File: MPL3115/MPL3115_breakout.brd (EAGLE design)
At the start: 15.2 x 11.2 mm, 2 parts

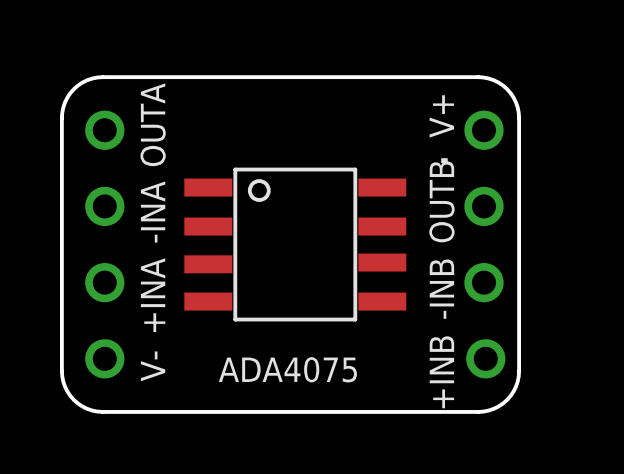
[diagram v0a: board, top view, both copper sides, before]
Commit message: Update new meme.
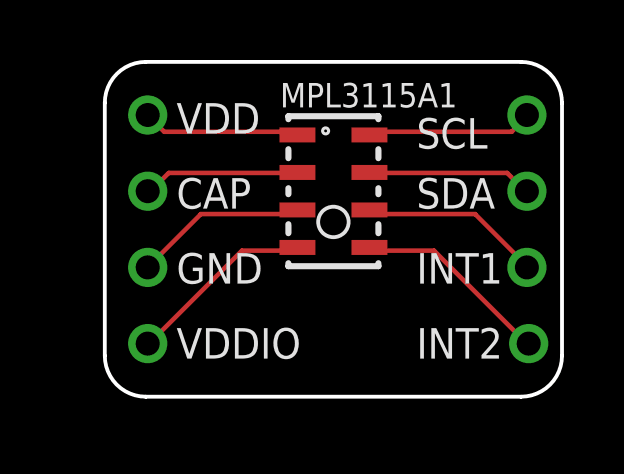
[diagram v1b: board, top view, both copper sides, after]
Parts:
- removed .: ADA4075, FaBo-Opamp:SOIC(NARROW)-8
- removed U$3: 8PIN, FaBo-Breakout:8PIN
- added MPL3115A1: FS-MPL3115A2, FaBo-Mems:FREESCALE-MPL3115A2
- added U$1: 8PIN, FaBo-Breakout:8PIN
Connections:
- removed net 1: ..1, U$3.1
- removed net 2: ..2, U$3.2
- removed net 3: ..3, U$3.3
- removed net 4: ..4, U$3.4
- removed net 5: ..5, U$3.5
- removed net 6: ..6, U$3.6
- removed net 7: ..7, U$3.7
- removed net 8: ..8, U$3.8
- new net CAP: MPL3115A1.2, U$1.2
- new net GND: MPL3115A1.3, U$1.3
- new net INT1: MPL3115A1.6, U$1.6
- new net INT2: MPL3115A1.5, U$1.5
- new net SCL: MPL3115A1.8, U$1.8
- new net SDA: MPL3115A1.7, U$1.7
- new net VDD: MPL3115A1.1, U$1.1
- new net VDDIO: MPL3115A1.4, U$1.4
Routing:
- net INT2: track 0.00 -> 6.67 mm
- net VDDIO: track 0.00 -> 6.35 mm
- net INT1: track 0.00 -> 6.13 mm
- net GND: track 0.00 -> 5.85 mm
- net SCL: track 0.00 -> 5.59 mm
- net SDA: track 0.00 -> 5.51 mm
- net VDD: track 0.00 -> 5.31 mm
- net CAP: track 0.00 -> 5.25 mm
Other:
- board text added: "CAP"
- board text added: "GND"
- board text added: "INT1"
- board text added: "INT2"
- board text added: "SCL"
- board text added: "SDA"
- board text added: "VDD"
- board text added: "VDDIO"
- board text removed: "+INA"
- board text removed: "+INB"
- board text removed: "-INA"
- board text removed: "-INB"
- board text removed: "ADA4075"
- board text removed: "OUTA"
- board text removed: "OUTB"
- board text removed: "V+"
- board text removed: "V-"
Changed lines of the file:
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@@
 <setting verticaltext="up"/>
 </settings>
-<grid distance="0.25" unitdist="mm" unit="mm" style="lines" multiple="1" display="yes" altdistance="0.025" altunitdist="inch" altunit="inch"/>
+<grid distance="0.5" unitdist="mm" unit="mm" style="lines" multiple="1" display="yes" altdistance="0.025" altunitdist="inch" altunit="inch"/>
 <layers>
 <layer number="1" name="Top" color="4" fill="1" visible="yes" active="yes"/>
@@
 <layer number="49" name="Reference" color="7" fill="1" visible="yes" active="yes"/>
 <layer number="50" name="dxf" color="7" fill="1" visible="no" active="no"/>
-<layer number="51" name="tDocu" color="14" fill="1" visible="yes" active="yes"/>
+<layer number="51" name="tDocu" color="7" fill="1" visible="yes" active="yes"/>
 <layer number="52" name="bDocu" color="7" fill="1" visible="yes" active="yes"/>
 <layer number="53" name="tGND_GNDA" color="7" fill="9" visible="no" active="no"/>
@@
 <layer number="154" name="FabDoc2" color="2" fill="1" visible="no" active="no"/>
 <layer number="155" name="FabDoc3" color="7" fill="15" visible="no" active="no"/>
-<layer number="160" name="O_Dim" color="12" fill="11" visible="yes" active="yes"/>
 <layer number="199" name="Contour" color="7" fill="1" visible="yes" active="yes"/>
-<layer number="200" name="200bmp" color="1" fill="10" visible="yes" active="yes"/>
+<layer number="200" name="200bmp" color="1" fill="10" visible="no" active="yes"/>
 <layer number="201" name="201bmp" color="2" fill="1" visible="no" active="no"/>
 <layer number="202" name="202bmp" color="3" fill="1" visible="no" active="no"/>
@@
 <board>
 <plain>
-<text x="3.794" y="1.262" size="0.8128" layer="21">ADA4075</text>
-<text x="2.016" y="8.398" size="0.8128" layer="21" rot="R90">OUTA</text>
-<text x="2.016" y="5.858" size="0.8128" layer="21" rot="R90">-INA</text>
-<text x="2.016" y="2.818" size="0.8128" layer="21" rot="R90">+INA</text>
-<text x="11.64" y="9.398" size="0.8128" layer="21" rot="R90">V+</text>
-<text x="11.644" y="5.858" size="0.8128" layer="21" rot="R90">OUTB</text>
-<text x="11.644" y="3.318" size="0.8128" layer="21" rot="R90">-INB</text>
-<text x="11.644" y="0.278" size="0.8128" layer="21" rot="R90">+INB</text>
-<text x="2.016" y="1.278" size="0.8128" layer="21" rot="R90">V-</text>
+<text x="2.39" y="9.54" size="1.016" layer="21">VDD</text>
+<text x="2.39" y="7.04" size="1.016" layer="21">CAP</text>
+<text x="2.39" y="4.54" size="1.016" layer="21">GND</text>
+<text x="2.39" y="2.04" size="1.016" layer="21">VDDIO</text>
+<text x="10.39" y="2.04" size="1.016" layer="21">INT2</text>
+<text x="10.39" y="4.54" size="1.016" layer="21">INT1</text>
+<text x="10.39" y="7.04" size="1.016" layer="21">SDA</text>
+<text x="10.39" y="9.04" size="1.016" layer="21">SCL</text>
 </plain>
 <attributes>
@@
 </class>
 </classes>
-<designrules name="Elecrow_2-layer_eagle_rule">
+<designrules name="SeeedStudio_2layer_DRU_no_angle_20140221">
 <description language="de">&lt;b&gt;EAGLE Design Rules&lt;/b&gt;
 &lt;p&gt;
@@
 necessary adjustments and save your customized
 design rules under a new name.</description>
-<description language="zh">&lt;b&gt;Elecrow EAGLE Design Rules&lt;/b&gt;
+<description language="zh">&lt;b&gt;Seeed Studio EAGLE Design Rules&lt;/b&gt;
 </description>
 <param name="layerSetup" value="(1*16)"/>
-<param name="mtCopper" value="0.035mm 0.035mm 0.035mm 0.035mm 0.035mm 0.035mm 0.035mm 0.035mm 0.035mm 0.035mm 0.035mm 0.035mm 0.035mm 0.035mm 0.035mm 0.035mm"/>
-<param name="mtIsolate" value="1.5mm 0.15mm 0.2mm 0.15mm 0.2mm 0.15mm 0.2mm 0.15mm 0.2mm 0.15mm 0.2mm 0.15mm 0.2mm 0.15mm 0.2mm"/>
+<param name="mtCopper" value="0.035mm 0.0175mm 0.035mm 0.035mm 0.035mm 0.035mm 0.035mm 0.035mm 0.035mm 0.035mm 0.035mm 0.035mm 0.035mm 0.035mm 0.0175mm 0.035mm"/>
+<param name="mtIsolate" value="1.5mm 1.1mm 0.2mm 0.15mm 0.2mm 0.15mm 0.2mm 0.15mm 0.2mm 0.15mm 0.2mm 0.15mm 0.2mm 0.15mm 0.2mm"/>
 <param name="mdWireWire" value="6mil"/>
 <param name="mdWirePad" value="6mil"/>
@@
 </autorouter>
 <elements>
-<element name="U$3" library="FaBo-Breakout" package="8PIN" value="8PIN" x="7.46" y="5.842"/>
-<element name="." library="FaBo-Opamp" package="SOIC(NARROW)-8" value="ADA4075" x="6.35" y="5.842" rot="R270"/>
+<element name="MPL3115A1" library="FaBo-Mems" package="FREESCALE-MPL3115A2" value="FS-MPL3115A2" x="7.62" y="7.62"/>
+<element name="U$1" library="FaBo-Breakout" package="8PIN" value="8PIN" x="8.89" y="6.35"/>
 </elements>
 <signals>
-<signal name="1">
-<contactref element="U$3" pad="1"/>
-<contactref element="." pad="1"/>
-<wire x1="3.45" y1="7.742" x2="0" y2="9.652" width="0" layer="19" extent="1-1"/>
-</signal>
-<signal name="2">
-<contactref element="U$3" pad="2"/>
-<contactref element="." pad="2"/>
-<wire x1="0" y1="7.112" x2="3.45" y2="6.442" width="0" layer="19" extent="1-1"/>
-</signal>
-<signal name="3">
-<contactref element="U$3" pad="3"/>
-<contactref element="." pad="3"/>
-<wire x1="0" y1="4.572" x2="3.45" y2="5.182" width="0" layer="19" extent="1-1"/>
-</signal>
-<signal name="4">
-<contactref element="U$3" pad="4"/>
-<contactref element="." pad="4"/>
-<wire x1="0" y1="2.032" x2="3.45" y2="3.942" width="0" layer="19" extent="1-1"/>
-</signal>
-<signal name="8">
-<contactref element="U$3" pad="8"/>
-<contactref element="." pad="8"/>
-<wire x1="9.25" y1="7.742" x2="12.64" y2="9.652" width="0" layer="19" extent="1-1"/>
-</signal>
-<signal name="7">
-<contactref element="U$3" pad="7"/>
-<contactref element="." pad="7"/>
-<wire x1="9.25" y1="6.442" x2="12.64" y2="7.112" width="0" layer="19" extent="1-1"/>
-</signal>
-<signal name="6">
-<contactref element="U$3" pad="6"/>
-<contactref element="." pad="6"/>
-<wire x1="9.25" y1="5.242" x2="12.64" y2="4.572" width="0" layer="19" extent="1-1"/>
-</signal>
-<signal name="5">
-<contactref element="U$3" pad="5"/>
-<contactref element="." pad="5"/>
-<wire x1="12.7" y1="2.032" x2="9.25" y2="3.942" width="0" layer="19" extent="1-1"/>
+<signal name="VDD">
+<contactref element="U$1" pad="1"/>
+<contactref element="MPL3115A1" pad="1"/>
+<wire x1="1.9812" y1="9.6012" x2="6.4008" y2="9.6012" width="0.1524" layer="1"/>
+<wire x1="1.524" y1="10.0584" x2="1.9812" y2="9.6012" width="0.1524" layer="1"/>
+<wire x1="6.4008" y1="9.6012" x2="6.42" y2="9.495" width="0.1524" layer="1"/>
+<wire x1="1.524" y1="10.0584" x2="1.43" y2="10.16" width="0.1524" layer="1"/>
+</signal>
+<signal name="CAP">
+<contactref element="U$1" pad="2"/>
+<contactref element="MPL3115A1" pad="2"/>
+<wire x1="2.1336" y1="8.2296" x2="6.4008" y2="8.2296" width="0.1524" layer="1"/>
+<wire x1="1.524" y1="7.62" x2="2.1336" y2="8.2296" width="0.1524" layer="1"/>
+<wire x1="6.4008" y1="8.2296" x2="6.42" y2="8.245" width="0.1524" layer="1"/>
+<wire x1="1.524" y1="7.62" x2="1.43" y2="7.62" width="0.1524" layer="1"/>
+</signal>
+<signal name="GND">
+<contactref element="U$1" pad="3"/>
+<contactref element="MPL3115A1" pad="3"/>
+<wire x1="3.2004" y1="6.858" x2="6.4008" y2="6.858" width="0.1524" layer="1"/>
+<wire x1="1.524" y1="5.1816" x2="3.2004" y2="6.858" width="0.1524" layer="1"/>
+<wire x1="6.4008" y1="6.858" x2="6.42" y2="6.995" width="0.1524" layer="1"/>
+<wire x1="1.524" y1="5.1816" x2="1.43" y2="5.08" width="0.1524" layer="1"/>
+</signal>
+<signal name="VDDIO">
+<contactref element="U$1" pad="4"/>
+<contactref element="MPL3115A1" pad="4"/>
+<wire x1="4.572" y1="5.6388" x2="6.4008" y2="5.6388" width="0.1524" layer="1"/>
+<wire x1="1.524" y1="2.5908" x2="4.572" y2="5.6388" width="0.1524" layer="1"/>
+<wire x1="6.4008" y1="5.6388" x2="6.42" y2="5.745" width="0.1524" layer="1"/>
+<wire x1="1.524" y1="2.5908" x2="1.43" y2="2.54" width="0.1524" layer="1"/>
+</signal>
+<signal name="SCL">
+<contactref element="U$1" pad="8"/>
+<contactref element="MPL3115A1" pad="8"/>
+<wire x1="13.5636" y1="9.6012" x2="8.8392" y2="9.6012" width="0.1524" layer="1"/>
+<wire x1="14.0208" y1="10.0584" x2="13.5636" y2="9.6012" width="0.1524" layer="1"/>
+<wire x1="8.8392" y1="9.6012" x2="8.82" y2="9.495" width="0.1524" layer="1"/>
+<wire x1="14.0208" y1="10.0584" x2="14.07" y2="10.16" width="0.1524" layer="1"/>
+</signal>
+<signal name="SDA">
+<contactref element="U$1" pad="7"/>
+<contactref element="MPL3115A1" pad="7"/>
+<wire x1="13.4112" y1="8.2296" x2="8.8392" y2="8.2296" width="0.1524" layer="1"/>
+<wire x1="14.0208" y1="7.62" x2="13.4112" y2="8.2296" width="0.1524" layer="1"/>
+<wire x1="8.8392" y1="8.2296" x2="8.82" y2="8.245" width="0.1524" layer="1"/>
+<wire x1="14.0208" y1="7.62" x2="14.07" y2="7.62" width="0.1524" layer="1"/>
+</signal>
+<signal name="INT1">
+<contactref element="U$1" pad="6"/>
+<contactref element="MPL3115A1" pad="6"/>
+<wire x1="12.3444" y1="6.858" x2="8.8392" y2="6.858" width="0.1524" layer="1"/>
+<wire x1="14.0208" y1="5.1816" x2="12.3444" y2="6.858" width="0.1524" layer="1"/>
+<wire x1="8.8392" y1="6.858" x2="8.82" y2="6.995" width="0.1524" layer="1"/>
+<wire x1="14.0208" y1="5.1816" x2="14.07" y2="5.08" width="0.1524" layer="1"/>
+</signal>
+<signal name="INT2">
+<contactref element="U$1" pad="5"/>
+<contactref element="MPL3115A1" pad="5"/>
+<wire x1="10.9728" y1="5.6388" x2="8.8392" y2="5.6388" width="0.1524" layer="1"/>
+<wire x1="14.0208" y1="2.5908" x2="10.9728" y2="5.6388" width="0.1524" layer="1"/>
+<wire x1="8.8392" y1="5.6388" x2="8.82" y2="5.745" width="0.1524" layer="1"/>
+<wire x1="14.0208" y1="2.5908" x2="14.13" y2="2.54" width="0.1524" layer="1"/>
 </signal>
 </signals>
-<errors>
-</errors>
 </board>
 </drawing>
